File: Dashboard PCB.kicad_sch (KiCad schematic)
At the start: 33 parts, among them J1 Controls_Leader_Export_02x06, J4 FAN_CTRL_01x02, J5 Horn_In_01x02, J6 Horn_Out_01x02

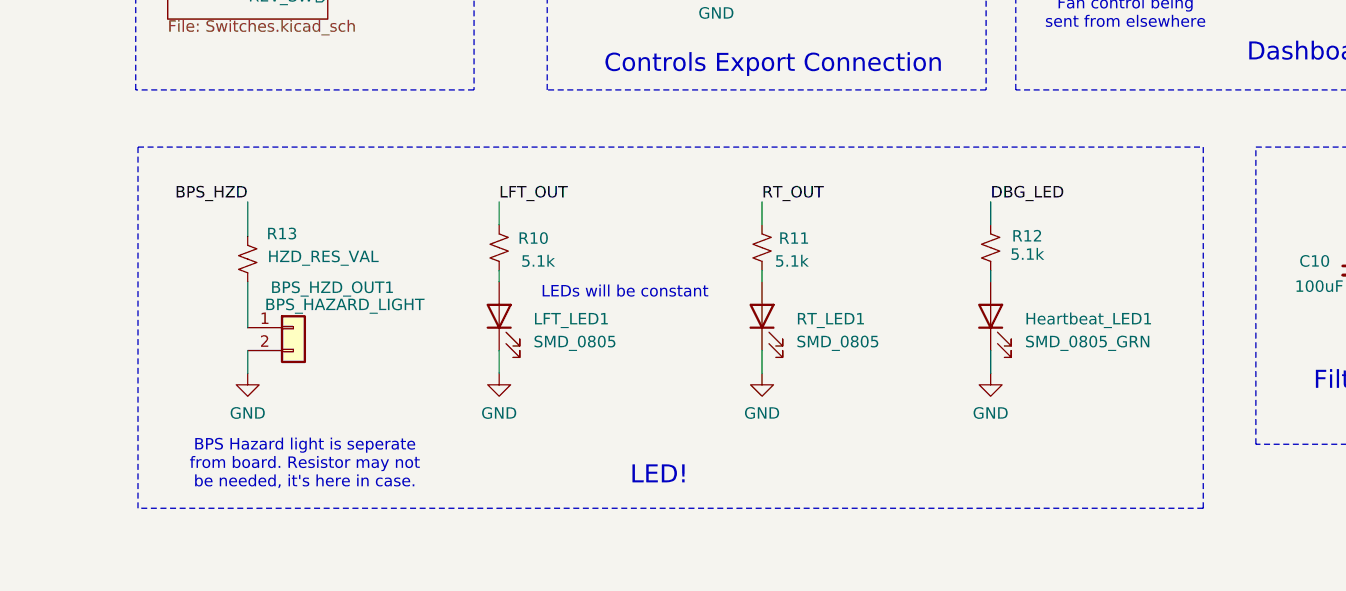
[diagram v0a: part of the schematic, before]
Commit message: r pt 2
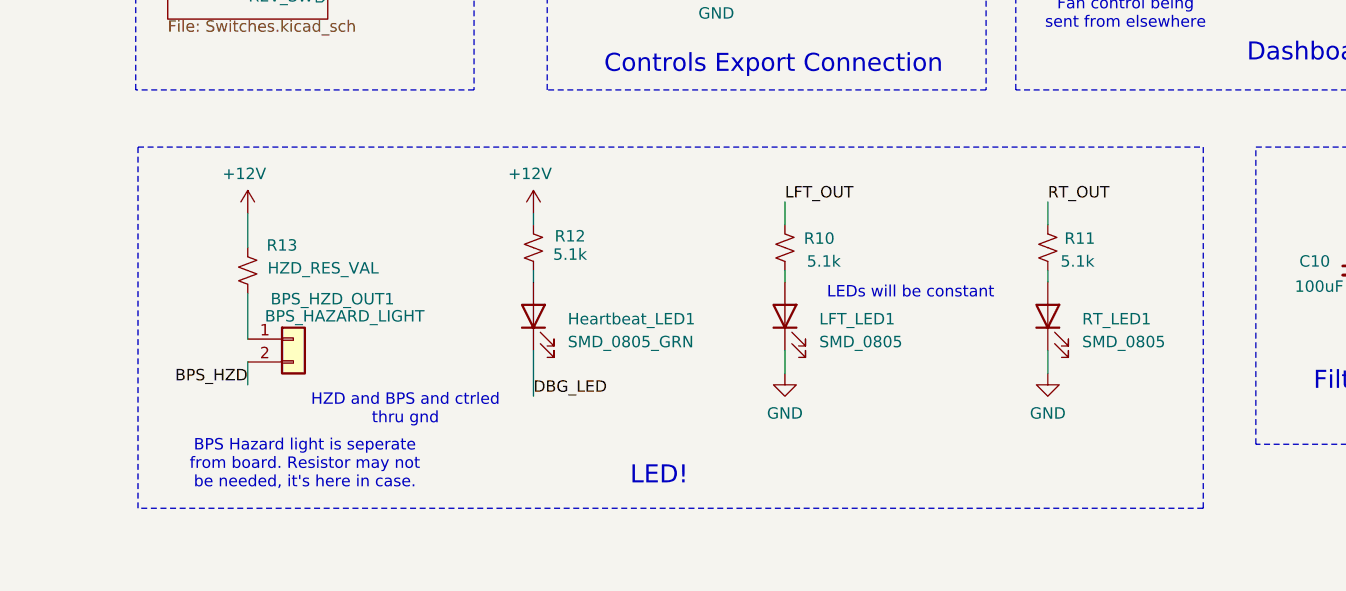
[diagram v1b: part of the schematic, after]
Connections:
- net +12V: now also R12.1, R13.1
- net BPS_HZD: now also BPS_HZD_OUT1.2 (Pin_2); no longer R13.1
- net DBG_LED: now also Heartbeat_LED1.1 (K); no longer R12.1
- net GND: no longer BPS_HZD_OUT1.2 (Pin_2), Heartbeat_LED1.1 (K)
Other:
- note added: "HZD and BPS and ctrled thru gnd"
- moved on the sheet: BPS_HZD_OUT1, Heartbeat_LED1, LFT_LED1, R10, R11, R12, R13, RT_LED1
